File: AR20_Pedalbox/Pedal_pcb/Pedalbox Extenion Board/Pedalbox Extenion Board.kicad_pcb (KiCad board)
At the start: 2 copper layers, 4 parts, among them P1 MX23A12NF1, U1 ACM_2020, U2 L78L05_SO8, U3 L78L05_SO8

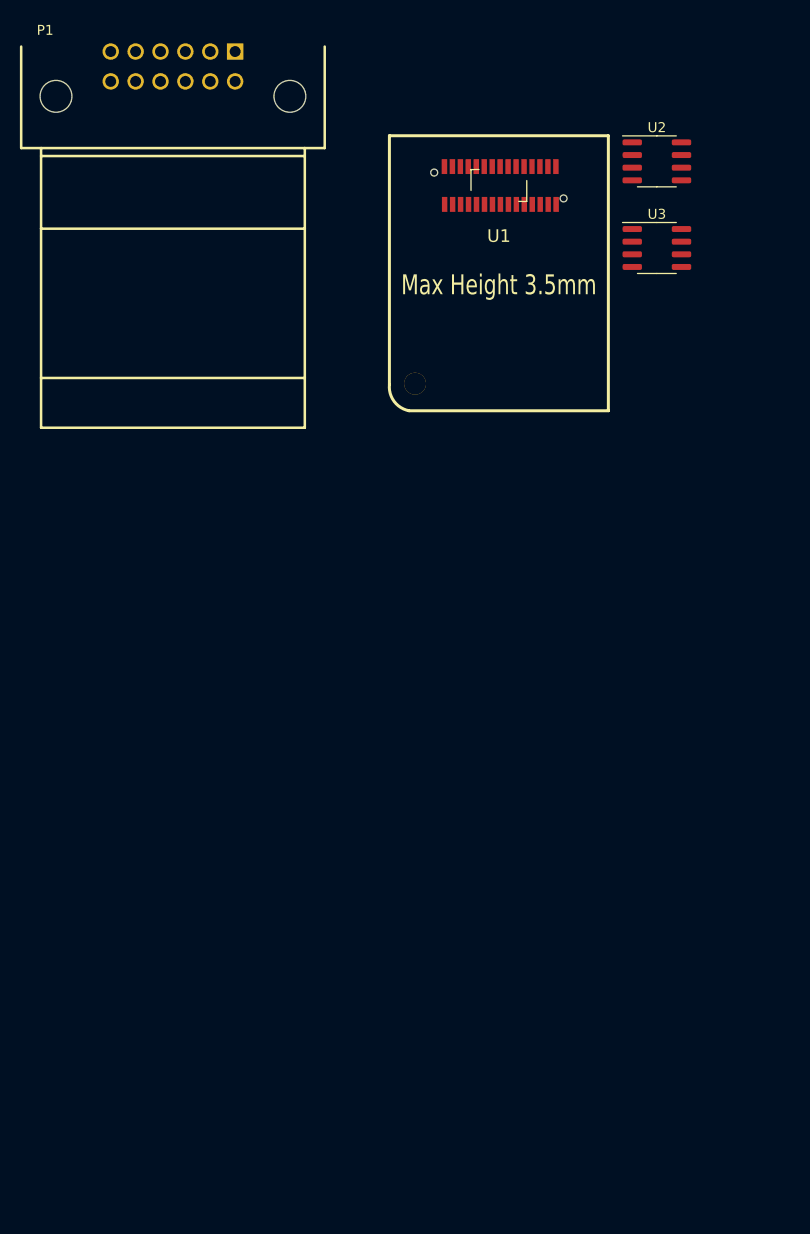
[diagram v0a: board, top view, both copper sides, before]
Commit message: Started on PCB layout and added 18pin connector
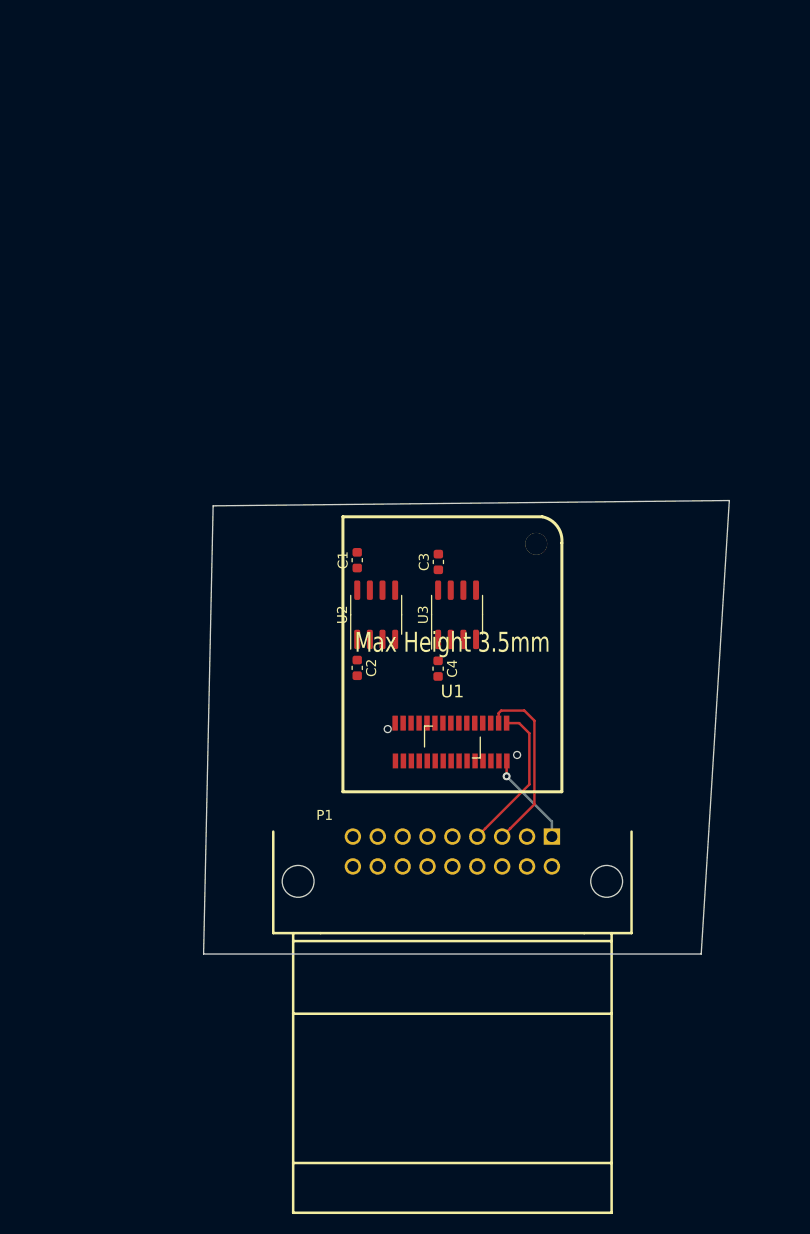
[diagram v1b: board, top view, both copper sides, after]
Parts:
- added C1: 0.33uF, Capacitor_SMD:C_0603_1608Metric, F.Cu at (140.4, 117.7)
- added C2: 0.1uF, Capacitor_SMD:C_0603_1608Metric, F.Cu at (140.4, 128.5)
- added C3: 0.33uF, Capacitor_SMD:C_0603_1608Metric, F.Cu at (148.6, 117.9)
- added C4: 0.1uF, Capacitor_SMD:C_0603_1608Metric, F.Cu at (148.6, 128.6)
- P1: value MX23A12NF1 -> MX23A18NF1; footprint Pedalbox Extenion Board:JAE_MX23A12NF1 -> MX23A18NF1:JAE_MX23A18NF1
- moved P1 83.7 mm to (150.0, 150.0)
- moved U1 56.1 mm to (150.0, 136.0), turned to 180 degrees
- moved U2 53.6 mm to (142.3, 123.2), turned to 90 degrees
- moved U3 42.0 mm to (150.5, 123.2), turned to 90 degrees
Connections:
- net Net-(P1-Pad10) renamed BPS2_Signal
- net Net-(P1-Pad11) renamed BPS1_Signal
- net Net-(P1-Pad8) renamed BPS2_Supply
- net Net-(P1-Pad9) renamed BPS2_GND
- P1 pad 1: Net-(P1-Pad1) -> +12V
- P1 pad 12: Net-(P1-Pad12) -> Steering_Angle_Sensor_Supply
- P1 pad 2: Net-(P1-Pad2) -> APPS1_GND
- P1 pad 3: Net-(P1-Pad3) -> CANH
- P1 pad 4: Net-(P1-Pad4) -> CANL
- P1 pad 5: Net-(P1-Pad5) -> Steering_Angle_Sensor_Supply
- P1 pad 6: Net-(P1-Pad6) -> APPS1_GND
- P1 pad 7: Net-(P1-Pad7) -> Steering_Angle_Sensor_Signal
- U1 pad 1: Net-(U1-Pad1) -> Steering_Angle_Sensor_Signal
- U1 pad 16: GND -> APPS1_GND
- U1 pad 18: GND -> APPS1_GND
- U1 pad 19: GND -> APPS1_GND
- U1 pad 2: Net-(U1-Pad2) -> APPS2_Signal
- U1 pad 21: GND -> APPS1_GND
- U1 pad 24: +5V -> Steering_Angle_Sensor_Supply
- U1 pad 26: Net-(U1-Pad26) -> Steering_Angle_Sensor_Supply
- U1 pad 27: Net-(U1-Pad27) -> CANH
- U1 pad 28: Net-(U1-Pad28) -> Steering_Angle_Sensor_Supply
- U1 pad 29: Net-(U1-Pad29) -> CANL
- U1 pad 3: Net-(U1-Pad3) -> APPS1_Signal
- U1 pad 9: GND -> APPS1_GND
- U2 pad 1: Net-(U2-Pad1) -> APPS1_Supply
- U2 pad 2: Net-(U2-Pad2) -> APPS1_GND
- U2 pad 3: Net-(U2-Pad2) -> APPS1_GND
- U2 pad 6: Net-(U2-Pad2) -> APPS1_GND
- U2 pad 7: Net-(U2-Pad2) -> APPS1_GND
- U2 pad 8: Net-(U2-Pad8) -> +12V
- U3 pad 1: Net-(U3-Pad1) -> APPS2_Supply
- U3 pad 2: Net-(U3-Pad2) -> APPS1_GND
- U3 pad 3: Net-(U3-Pad2) -> APPS1_GND
- U3 pad 6: Net-(U3-Pad2) -> APPS1_GND
- U3 pad 7: Net-(U3-Pad2) -> APPS1_GND
- U3 pad 8: Net-(U3-Pad8) -> +12V
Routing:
- net CANH: track 0.00 -> 18.1 mm
- net CANL: track 0.00 -> 15.3 mm
- net +12V: track 0.00 -> 9.50 mm, vias 0 -> 1
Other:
- board outline added: 52.8 x 45.6 mm

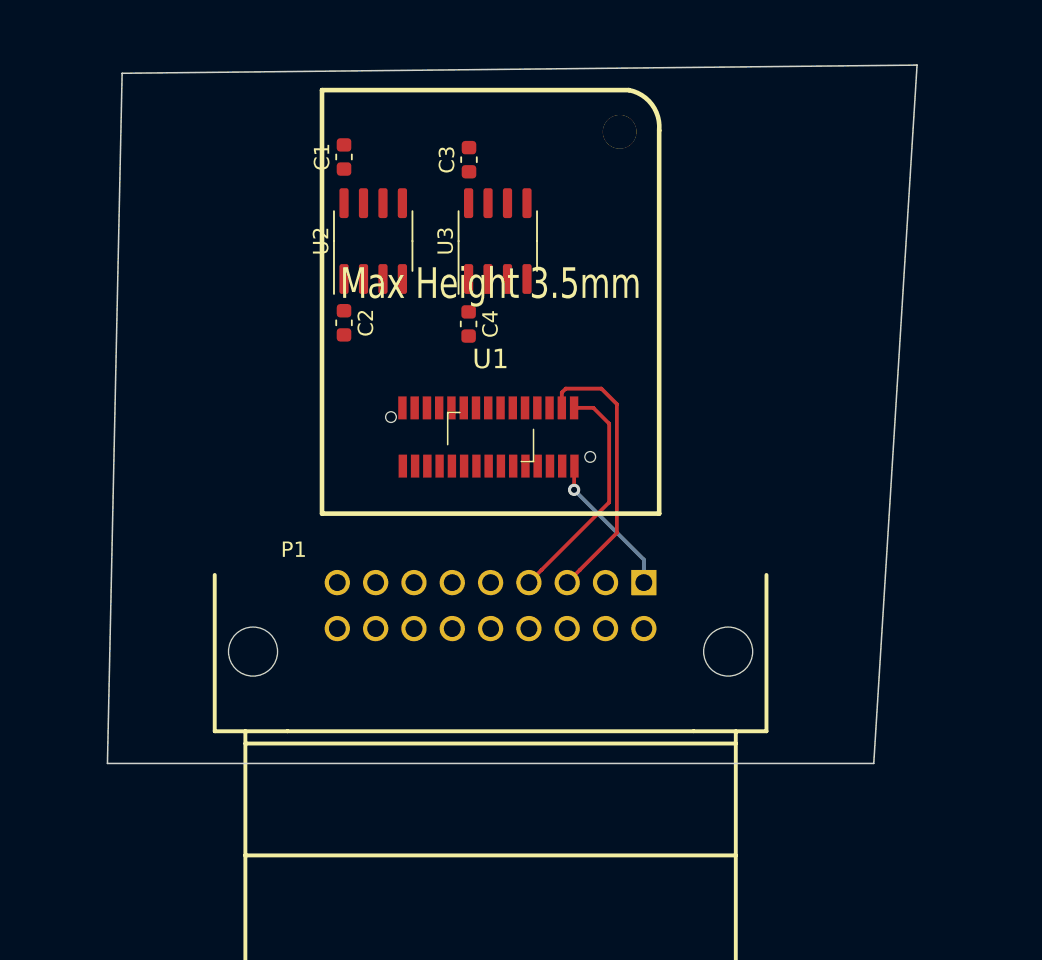
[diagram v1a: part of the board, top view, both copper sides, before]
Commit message: Pedalbox PCB Ready - Just need some more silkscreen... ;)
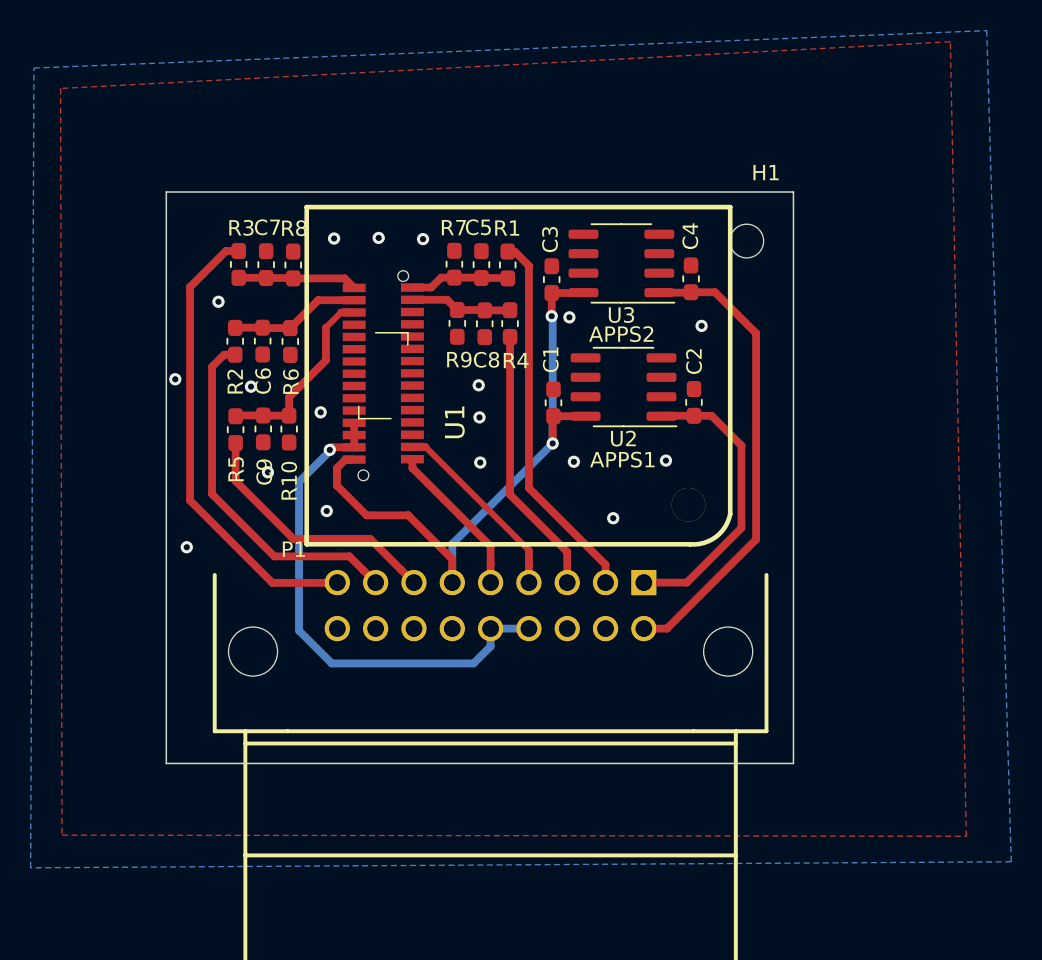
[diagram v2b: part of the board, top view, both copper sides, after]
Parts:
- added C5: C_Small, Capacitor_SMD:C_0603_1608Metric_Pad1.05x0.95mm_HandSolder, F.Cu at (149.4, 124.8)
- added C6: C_Small, Capacitor_SMD:C_0603_1608Metric_Pad1.05x0.95mm_HandSolder, F.Cu at (135.1, 129.7)
- added C7: C_Small, Capacitor_SMD:C_0603_1608Metric_Pad1.05x0.95mm_HandSolder, F.Cu at (135.4, 124.8)
- added C8: C_Small, Capacitor_SMD:C_0603_1608Metric_Pad1.05x0.95mm_HandSolder, F.Cu at (149.6, 128.6)
- added C9: C_Small, Capacitor_SMD:C_0603_1608Metric_Pad1.05x0.95mm_HandSolder, F.Cu at (135.2, 135.5)
- added H1: MountingHole, MountingHole:MountingHole_2.2mm_M2, F.Cu at (166.7, 123.2)
- added R1: R_Small, Resistor_SMD:R_0603_1608Metric_Pad1.05x0.95mm_HandSolder, F.Cu at (151.1, 124.8)
- added R10: 4K7, Resistor_SMD:R_0603_1608Metric_Pad1.05x0.95mm_HandSolder, F.Cu at (136.9, 135.5)
- added R2: R_Small, Resistor_SMD:R_0603_1608Metric_Pad1.05x0.95mm_HandSolder, F.Cu at (133.3, 129.8)
- added R3: R_Small, Resistor_SMD:R_0603_1608Metric_Pad1.05x0.95mm_HandSolder, F.Cu at (133.6, 124.7)
- added R4: R_Small, Resistor_SMD:R_0603_1608Metric_Pad1.05x0.95mm_HandSolder, F.Cu at (151.3, 128.6)
- added R5: R_Small, Resistor_SMD:R_0603_1608Metric_Pad1.05x0.95mm_HandSolder, F.Cu at (133.4, 135.5)
- added R6: 4K7, Resistor_SMD:R_0603_1608Metric_Pad1.05x0.95mm_HandSolder, F.Cu at (136.9, 129.8)
- added R7: 4K7, Resistor_SMD:R_0603_1608Metric_Pad1.05x0.95mm_HandSolder, F.Cu at (147.6, 124.7)
- added R8: 4K7, Resistor_SMD:R_0603_1608Metric_Pad1.05x0.95mm_HandSolder, F.Cu at (137.1, 124.8)
- added R9: 4K7, Resistor_SMD:R_0603_1608Metric_Pad1.05x0.95mm_HandSolder, F.Cu at (147.8, 128.6)
- C1, C2, C3, C4: footprint Capacitor_SMD:C_0603_1608Metric -> Capacitor_SMD:C_0603_1608Metric_Pad1.05x0.95mm_HandSolder
- moved C2 23.4 mm to (163.3, 133.7), turned to 90 degrees
- moved C1 21.1 mm to (154.1, 133.8)
- moved U2 18.9 mm to (158.7, 132.7), turned to 180 degrees
- moved C4 14.8 mm to (163.1, 125.7), turned to 90 degrees
- moved C3 9.50 mm to (154.0, 125.7)
- moved U3 8.20 mm to (158.5, 124.7), turned to 180 degrees
- moved U1 8.06 mm to (143.0, 132.0), turned to 90 degrees
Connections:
- C1 pad 2: APPS1_GND -> GND
- C2 pad 2: APPS1_GND -> GND
- C3 pad 2: APPS1_GND -> GND
- C4 pad 2: APPS1_GND -> GND
- P1 pad 1: +12V -> APPS1_Supply
- P1 pad 10: BPS2_Signal -> APPS2_Supply
- P1 pad 11: BPS1_Signal -> GND
- P1 pad 12: Steering_Angle_Sensor_Supply -> GND
- P1 pad 13: APPS2_Supply -> +5V
- P1 pad 14: APPS1_GND -> +5V
- P1 pad 15: APPS2_Signal -> GND
- P1 pad 16: APPS1_Supply -> GND
- P1 pad 17: APPS1_GND -> GND
- P1 pad 18: APPS1_Signal -> GND
- P1 pad 2: APPS1_GND -> APPS1_Signal
- P1 pad 3: CANH -> APPS2_Signal
- P1 pad 4: CANL -> CANH
- P1 pad 5: Steering_Angle_Sensor_Supply -> CANL
- P1 pad 6: APPS1_GND -> +12V
- P1 pad 7: Steering_Angle_Sensor_Signal -> BPS2_Signal
- P1 pad 8: BPS2_Supply -> BPS1_Signal
- P1 pad 9: BPS2_GND -> Steering_Angle_Sensor_Signal
- U1 pad 1: Steering_Angle_Sensor_Signal -> APPS1_Signal_Filtered
- U1 pad 16: APPS1_GND -> GND
- U1 pad 18: APPS1_GND -> GND
- U1 pad 19: APPS1_GND -> GND
- U1 pad 2: APPS2_Signal -> Steering_Angle_Sensor_Signal_Filtered
- U1 pad 21: APPS1_GND -> GND
- U1 pad 24: Steering_Angle_Sensor_Supply -> +5V
- U1 pad 26: Steering_Angle_Sensor_Supply -> +5V
- U1 pad 28: Steering_Angle_Sensor_Supply -> +5V
- U1 pad 3: APPS1_Signal -> APPS2_Signal_Filtered
- U1 pad 4: Net-(U1-Pad4) -> BPS1_Signal_Filtered
- U1 pad 6: Net-(U1-Pad6) -> BPS2_Signal_Filtered
- U1 pad 9: APPS1_GND -> GND
- U2 pad 2: APPS1_GND -> GND
- U2 pad 3: APPS1_GND -> GND
- U2 pad 6: APPS1_GND -> GND
- U2 pad 7: APPS1_GND -> GND
- U3 pad 2: APPS1_GND -> GND
- U3 pad 3: APPS1_GND -> GND
- U3 pad 6: APPS1_GND -> GND
- U3 pad 7: APPS1_GND -> GND
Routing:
- net +5V: track 0.00 -> 33.4 mm, vias 0 -> 1
- net +12V: track 9.50 -> 41.1 mm, vias 1 -> 2
- net APPS2_Supply: track 0.00 -> 30.6 mm
- net Steering_Angle_Sensor_Signal: track 0.00 -> 29.9 mm
- net APPS1_Signal: track 0.00 -> 24.5 mm
- net BPS1_Signal: track 0.00 -> 23.2 mm
- net APPS1_Supply: track 0.00 -> 19.3 mm
- net APPS2_Signal: track 0.00 -> 17.6 mm
- net BPS2_Signal: track 0.00 -> 16.9 mm
- net BPS2_Signal_Filtered: track 0.00 -> 12.5 mm
- net BPS1_Signal_Filtered: track 0.00 -> 8.53 mm
- net Steering_Angle_Sensor_Signal_Filtered: track 0.00 -> 7.81 mm
- net APPS2_Signal_Filtered: track 0.00 -> 6.66 mm
- net APPS1_Signal_Filtered: track 0.00 -> 6.51 mm
- net CANH: track 18.1 -> 12.5 mm
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- added copper zone on B.Cu, net GND
- added copper zone on F.Cu, net GND
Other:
- board size 52.8 x 45.6 mm -> 40.9 x 37.3 mm
- board text added: "APPS1"
- board text added: "APPS2"
- board text added: "Pedalbox Extention board Pedalbox Bachelor Thesis 2020 V. 1.0"
